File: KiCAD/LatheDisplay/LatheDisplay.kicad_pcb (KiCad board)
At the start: 2 copper layers, 80 x 86.4 mm, 38 parts, among them J1 Screw_Terminal_01x02, J2 Screw_Terminal_01x03, J3 AVR-ISP-6, J4 Conn_01x06_Pin, U1 D168K, U10 LM4040DBZ-4.1, U11 LM7812_TO220, U12 LM7912_TO220, U13 LM7805_TO220, U2 D168K, U3 D168K, U4 D168K, U5 D168K, U6 ICM7218B, U7 ATmega328-P, U8 TLC3541, U9 INA121

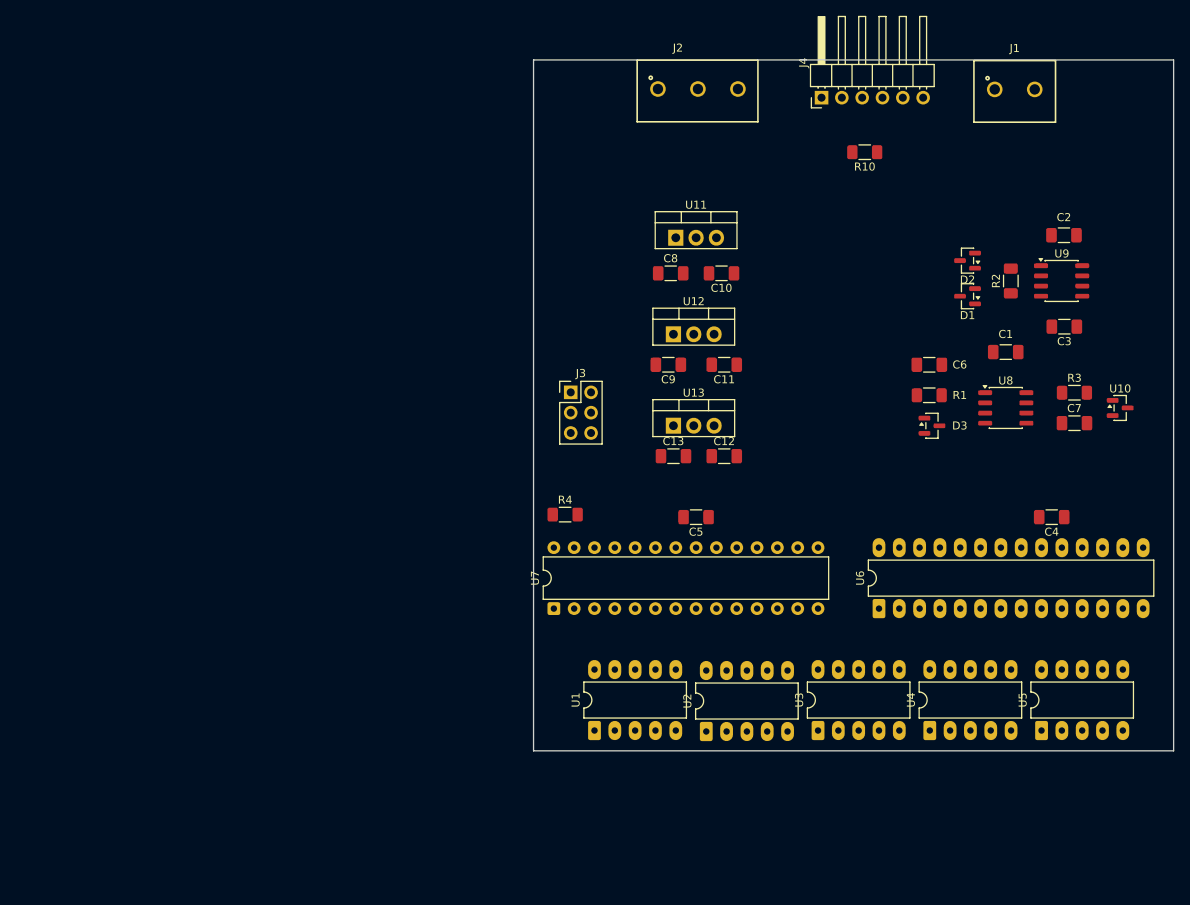
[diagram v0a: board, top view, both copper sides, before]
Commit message: save lathe stuff
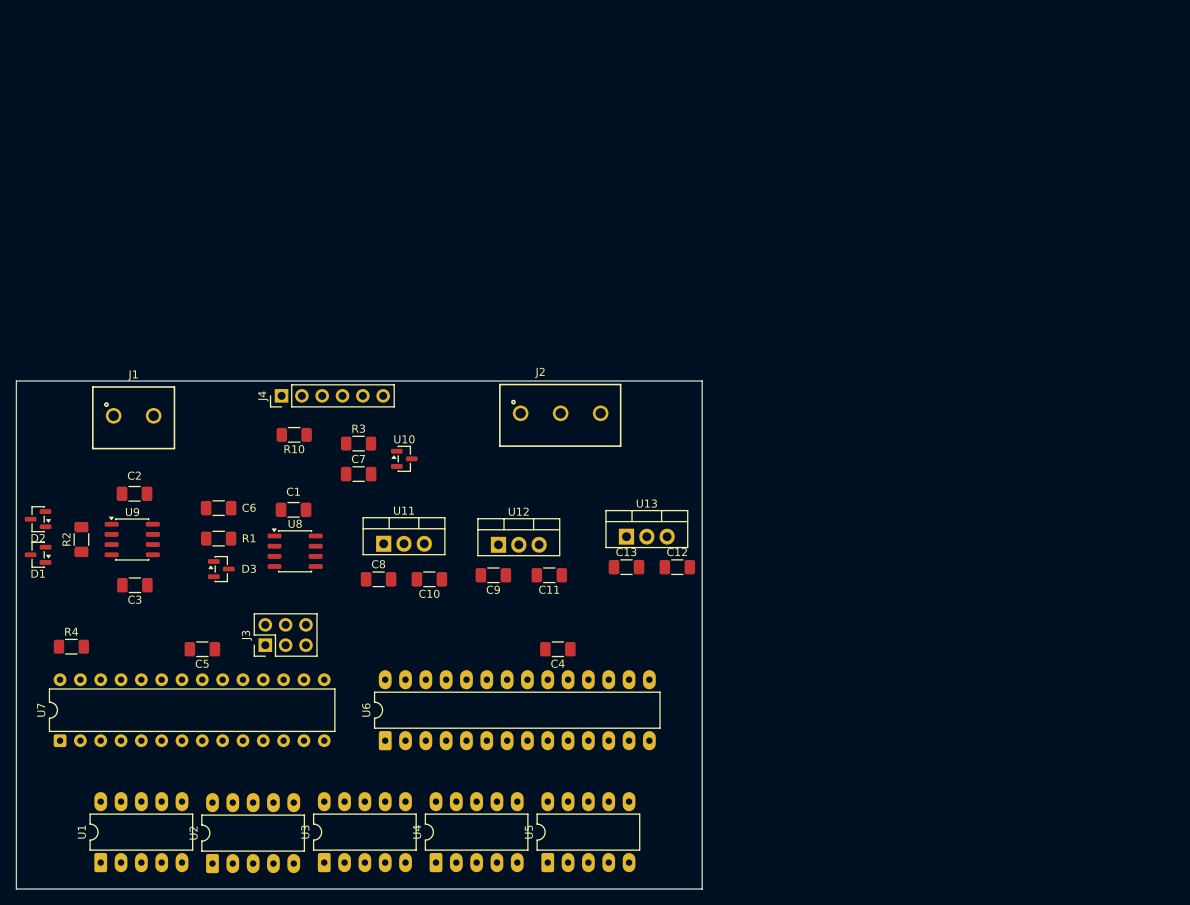
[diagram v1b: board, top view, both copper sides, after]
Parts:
- J4: footprint Connector_PinHeader_2.54mm:PinHeader_1x06_P2.54mm_Horizontal -> Connector_PinHeader_2.54mm:PinHeader_1x06_P2.54mm_Vertical
- R1: value 1k -> 2k
- moved D1 120.6 mm to (58.7, 101.2)
- moved D2 120.6 mm to (58.7, 96.8)
- moved C3 120.6 mm to (70.8, 105.0)
- moved R2 120.6 mm to (64.1, 99.3)
- moved U9 120.6 mm to (70.5, 99.3)
- moved C2 120.6 mm to (70.8, 93.6)
- moved J1 117.5 mm to (70.7, 83.8)
- moved C1 91.2 mm to (90.7, 95.6)
- moved C6 90.6 mm to (81.3, 95.4)
- moved R1 90.6 mm to (81.3, 99.2)
- moved U8 90.6 mm to (90.8, 100.8)
- moved D3 90.6 mm to (81.6, 103.0)
- moved C7 89.7 mm to (98.8, 91.1)
- moved R3 89.7 mm to (98.8, 87.3)
- moved U10 89.7 mm to (104.5, 89.2)
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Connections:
- R10 pad 1: VCC -> +5V
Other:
- board size 80 x 86.4 mm -> 85.7 x 63.5 mm
